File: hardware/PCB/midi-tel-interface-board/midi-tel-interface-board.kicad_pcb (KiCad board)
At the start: 2 copper layers, 145.5 x 48 mm, 17 parts, among them J1 DIN-5_180degree, J2 Conn_01x07_Male, J3 Conn_01x17_Male, J4 Conn_01x03, J5 Conn_01x03, J6 Conn_01x03, J7 Conn_01x03, SW1 SW_Push, U1 Pico

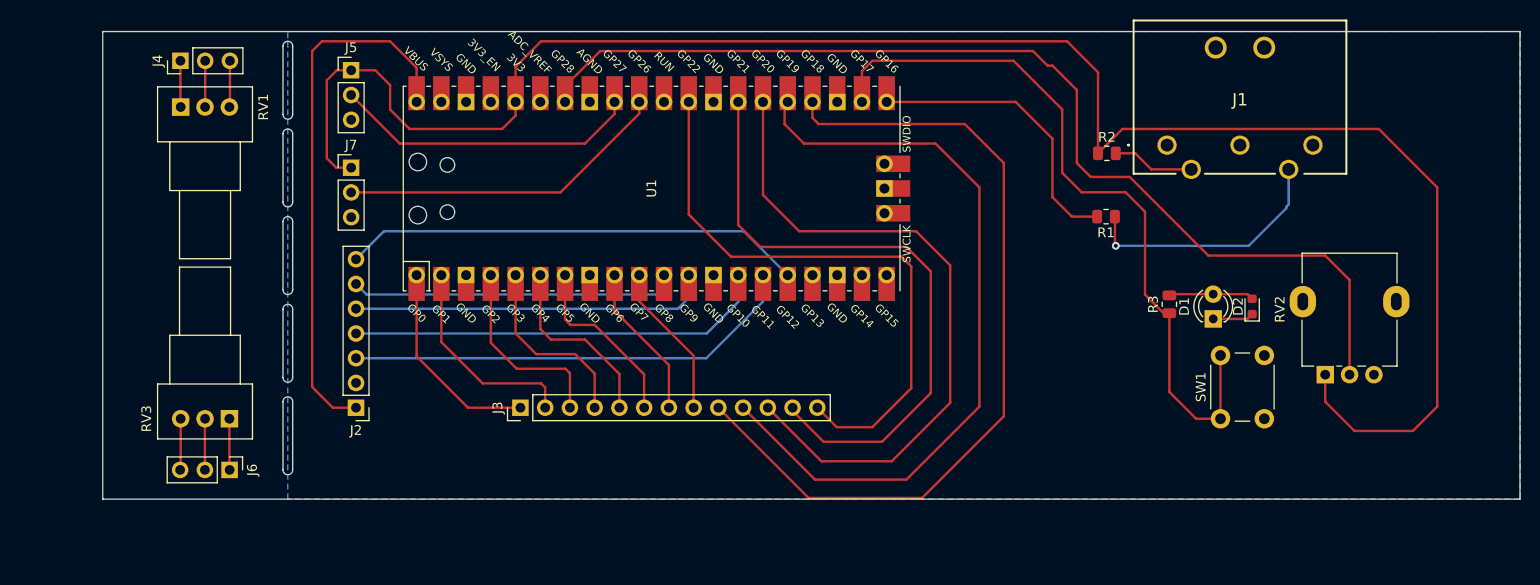
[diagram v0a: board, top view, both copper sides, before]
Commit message: update gitignore and pcb files
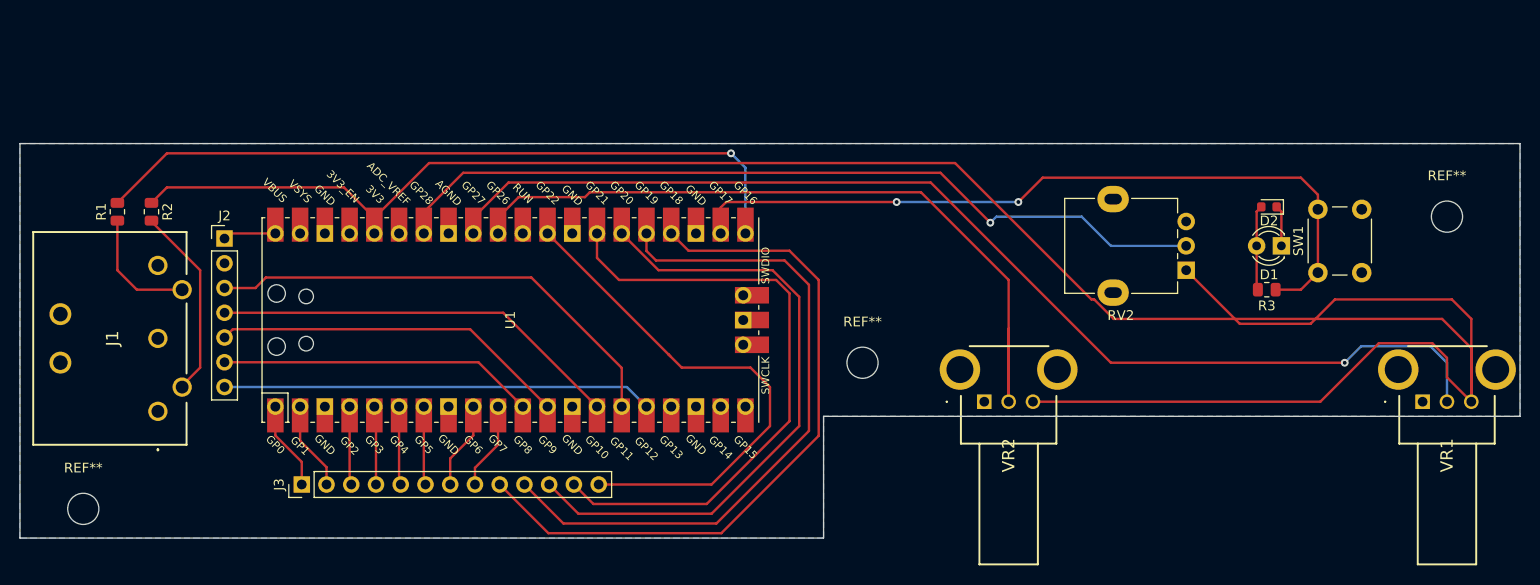
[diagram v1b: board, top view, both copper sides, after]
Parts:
- removed J4, J5, J6, J7: Conn_01x03, Connector_PinHeader_2.54mm:PinHeader_1x03_P2.54mm_Vertical
- removed RV1, RV3: R_Potentiometer, Potentiometer_THT:Potentiometer_Alps_RK09Y11_Single_Horizontal
- added REF**: MountingHole_3.2mm_M3, MountingHole:MountingHole_3.2mm_M3, F.Cu at (65.0, 80.0)
- added REF**: MountingHole_3.2mm_M3, MountingHole:MountingHole_3.2mm_M3, F.Cu at (205.0, 50.0)
- added REF**: MountingHole_3.2mm_M3, MountingHole:MountingHole_3.2mm_M3, F.Cu at (145.0, 65.0)
- added VR1: RK09K1110B26, RK09K1110B26:RK09K1110B26, F.Cu at (202.5, 69.0)
- added VR2: RK09K1110B26, RK09K1110B26:RK09K1110B26, F.Cu at (157.5, 69.0)
- moved J1 107.1 mm to (72.7, 70.0), turned to -90 degrees
- moved R1 101.5 mm to (68.5, 49.5), turned to 90 degrees
- moved R2 98.3 mm to (72.0, 49.5), turned to -90 degrees
- moved J3 23.8 mm to (87.4, 77.5)
- moved J2 22.0 mm to (79.5, 52.2), turned to 0 degrees
- moved U1 19.8 mm to (108.8, 60.6)
- moved SW1 18.0 mm to (191.8, 55.8)
- moved RV2 17.9 mm to (178.2, 55.5), turned to 180 degrees
- moved D2 10.4 mm to (186.7, 49.0), turned to 180 degrees
- moved D1 10.3 mm to (188.0, 53.0), turned to 180 degrees
- moved R3 10.1 mm to (186.5, 57.5), turned to 180 degrees
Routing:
- net /ADC_pitch: track 31.6 -> 116.1 mm, vias 0 -> 1
- net +3V3: track 188.2 -> 251.8 mm
- net +5V: track 55.6 -> 5.44 mm
- net /ADC_mode: track 34.1 -> 78.8 mm
- net /MIDI_out: track 30.0 -> 73.9 mm, vias 0 -> 1
- net /ADC_rate: track 107.5 -> 85.7 mm, vias 0 -> 1
- net /minitel_kb8: track 85.8 -> 72.1 mm
- net Net-(J1-Pad5): track 26.2 -> 12.6 mm, vias 1 -> 0
- net /minitel_kb1: track 21.5 -> 9.12 mm
- net /minitel_kb0: track 21.2 -> 9.12 mm
- net /minitel_kb2: track 19.9 -> 8.07 mm
- net Net-(J1-Pad4): track 8.43 -> 19.9 mm
- net /minitel_kb3: track 19.3 -> 8.07 mm
- net /minitel_kb4: track 19.0 -> 8.07 mm
- net /minitel_kb5: track 18.4 -> 8.07 mm
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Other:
- board size 145.5 x 48 mm -> 154 x 40.5 mm
